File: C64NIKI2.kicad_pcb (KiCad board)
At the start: 2 copper layers, 25 parts, among them J1 C64-EXP, Q1 BC237, SW1 FREEZE, SW2 RESET, U1 74LS74, U2 74LS163, U3 74LS125, U4 74LS05, U5 74LS174, U6 27C256

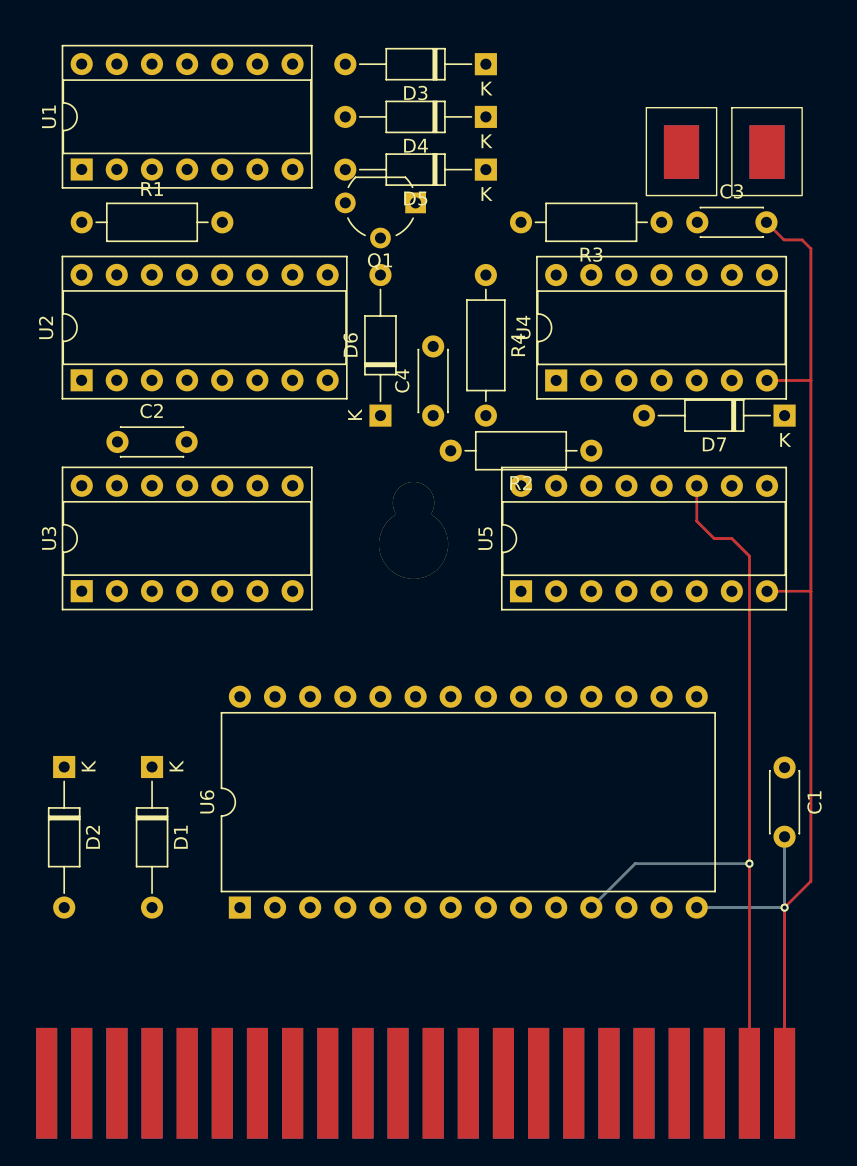
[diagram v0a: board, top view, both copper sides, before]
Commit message: complete net
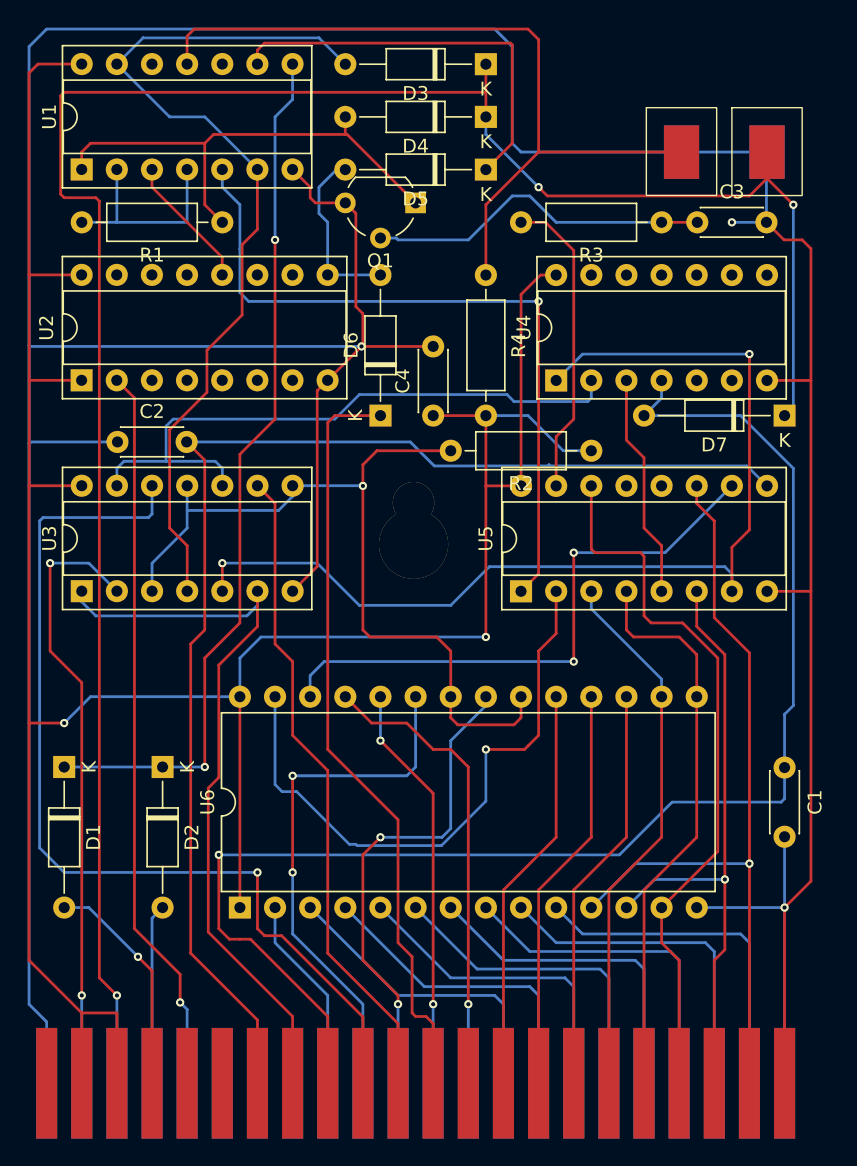
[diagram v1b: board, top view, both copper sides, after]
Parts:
- moved R1 10.2 mm to (106.7, 110.5), turned to 180 degrees
- moved D2 7.11 mm to (102.4, 149.9)
- moved D1 6.35 mm to (95.2, 149.9)
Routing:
- net GND: track 95.6 -> 312.0 mm, vias 1 -> 3
- net VCC: track 0.00 -> 213.4 mm, vias 0 -> 2
- net /EXP_C: track 0.00 -> 153.1 mm, vias 0 -> 3
- net /EXP_9: track 0.00 -> 102.8 mm, vias 0 -> 1
- net /EXP_7: track 0.00 -> 92.7 mm
- net Net-(U5-Q2): track 0.00 -> 75.2 mm, vias 0 -> 2
- net /EXP_10: track 0.00 -> 69.6 mm, vias 0 -> 1
- net Net-(D3-A): track 0.00 -> 65.0 mm
- net Net-(D1-K): track 0.00 -> 63.6 mm, vias 0 -> 2
- net Net-(U6-~{CE}): track 0.00 -> 60.1 mm, vias 0 -> 1
- net Net-(U1B-C): track 0.00 -> 56.9 mm
- net /BA: track 0.00 -> 55.4 mm
- net /EXP_8: track 0.00 -> 54.8 mm
- net /EXP_E: track 0.00 -> 52.9 mm, vias 0 -> 1
- net Net-(U1A-Q): track 0.00 -> 52.8 mm, vias 0 -> 1
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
